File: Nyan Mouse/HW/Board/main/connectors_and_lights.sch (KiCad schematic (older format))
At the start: 49 parts, among them Q301 MOSFET-NCHANNELSMD, Q302 MOSFET-NCHANNELSMD, Q303 MOSFET-PCHANNELSMD, Q304 MOSFET-NCHANNELSMD, Q305 MOSFET-PCHANNELSMD, Q306 MOSFET-NCHANNELSMD, Q307 MOSFET-PCHANNELSMD, Q308 MOSFET-NCHANNELSMD, Q309 MOSFET-NCHANNELSMD, Q310 MOSFET-NCHANNELSMD, Q311 MOSFET-NCHANNELSMD, Q312 MOSFET-NCHANNELSMD, U301 74HC595, U302 74HC595, U303 74HC595

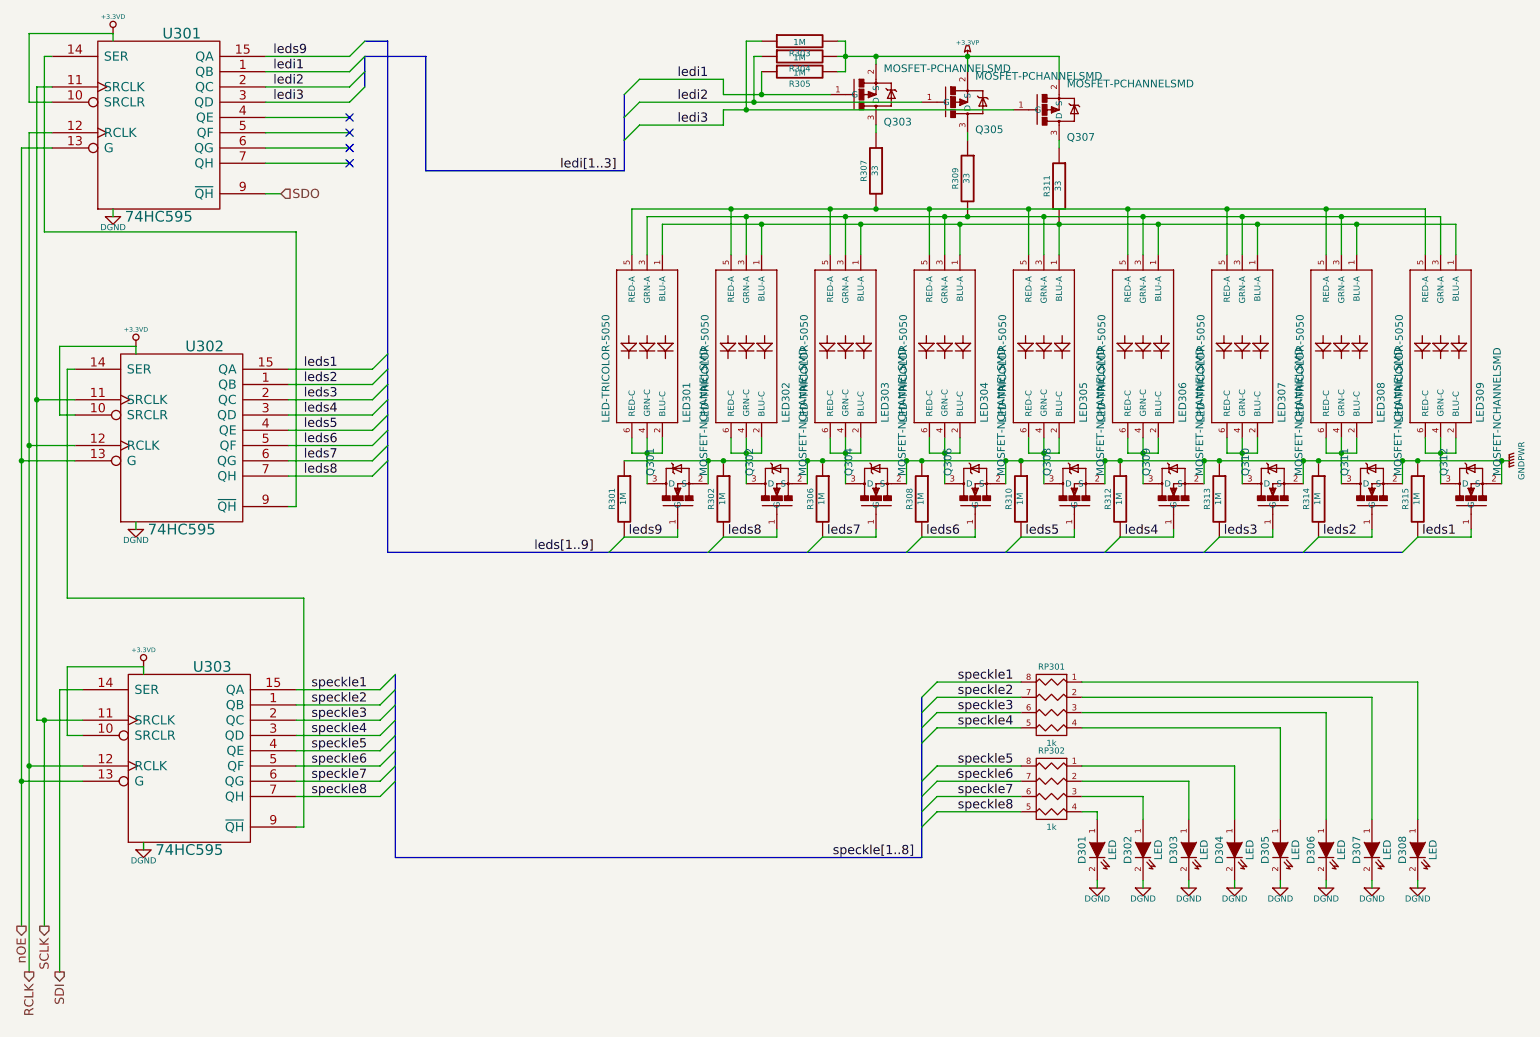
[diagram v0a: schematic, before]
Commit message: Updated schematics
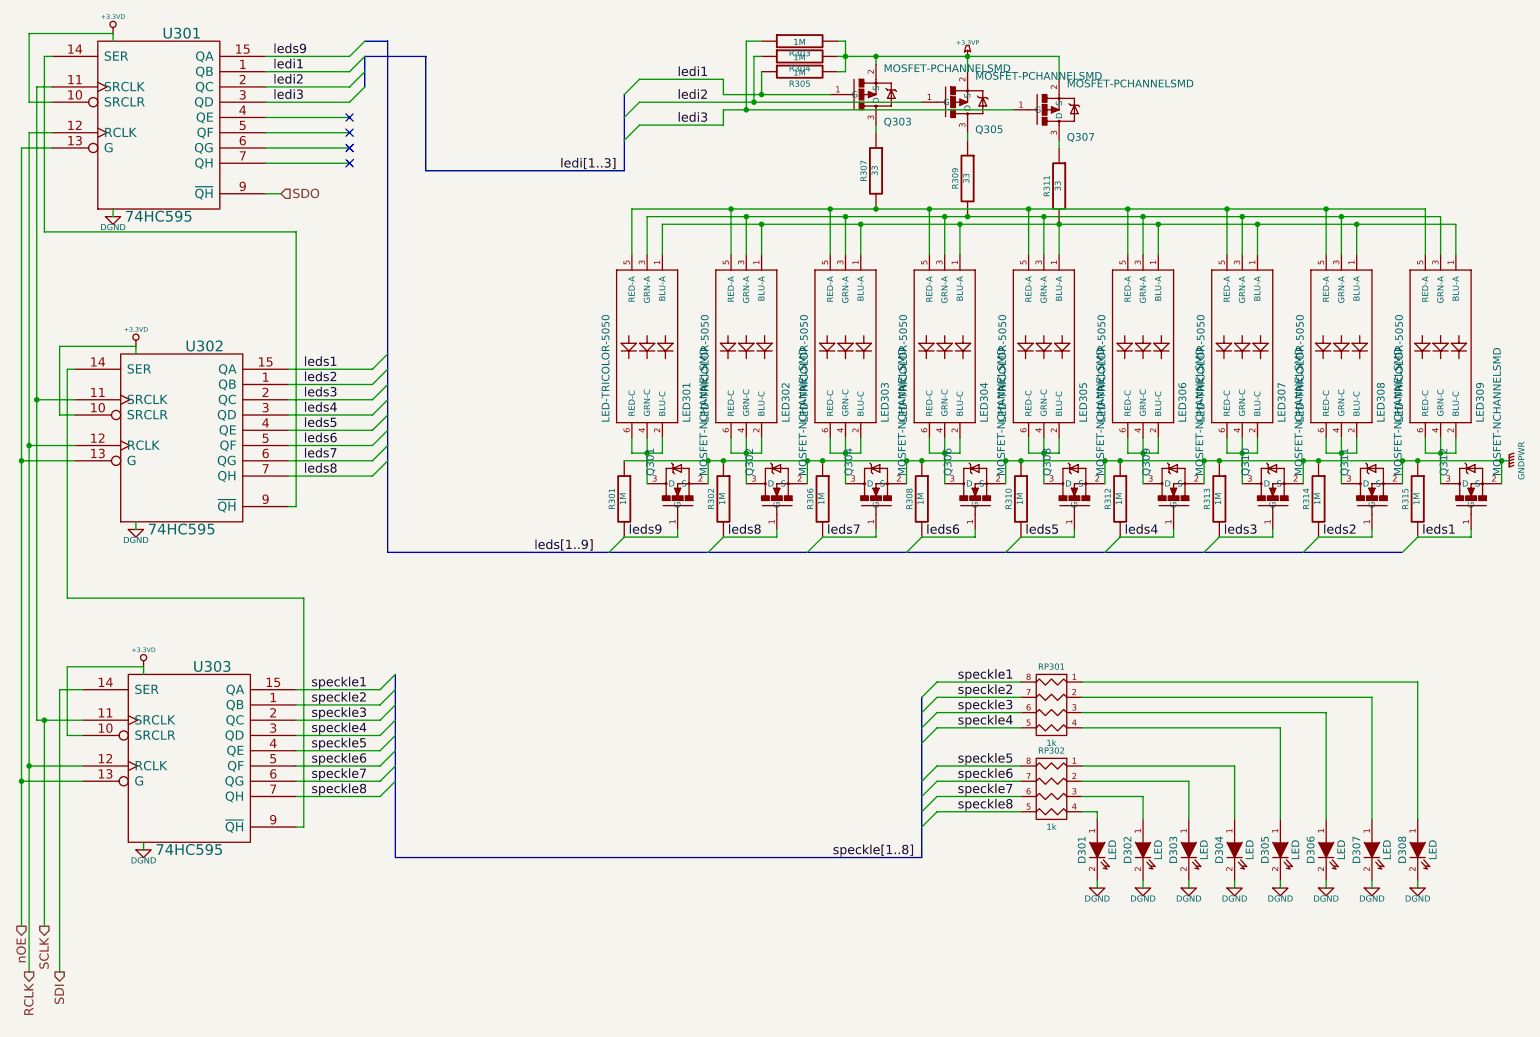
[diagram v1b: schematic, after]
